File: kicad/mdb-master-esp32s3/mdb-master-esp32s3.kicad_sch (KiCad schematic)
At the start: 40 parts, among them J2 MDB_Connector, J3 Barrel_Jack, J5 Conn_02x10_Odd_Even, P1 USB_C_Plug_USB2.0, Q1 BC807, SW1 Reset, SW2 Boot, U1 ESP32-S3FH4R2, U2 TS1117B, Y1 40000hz

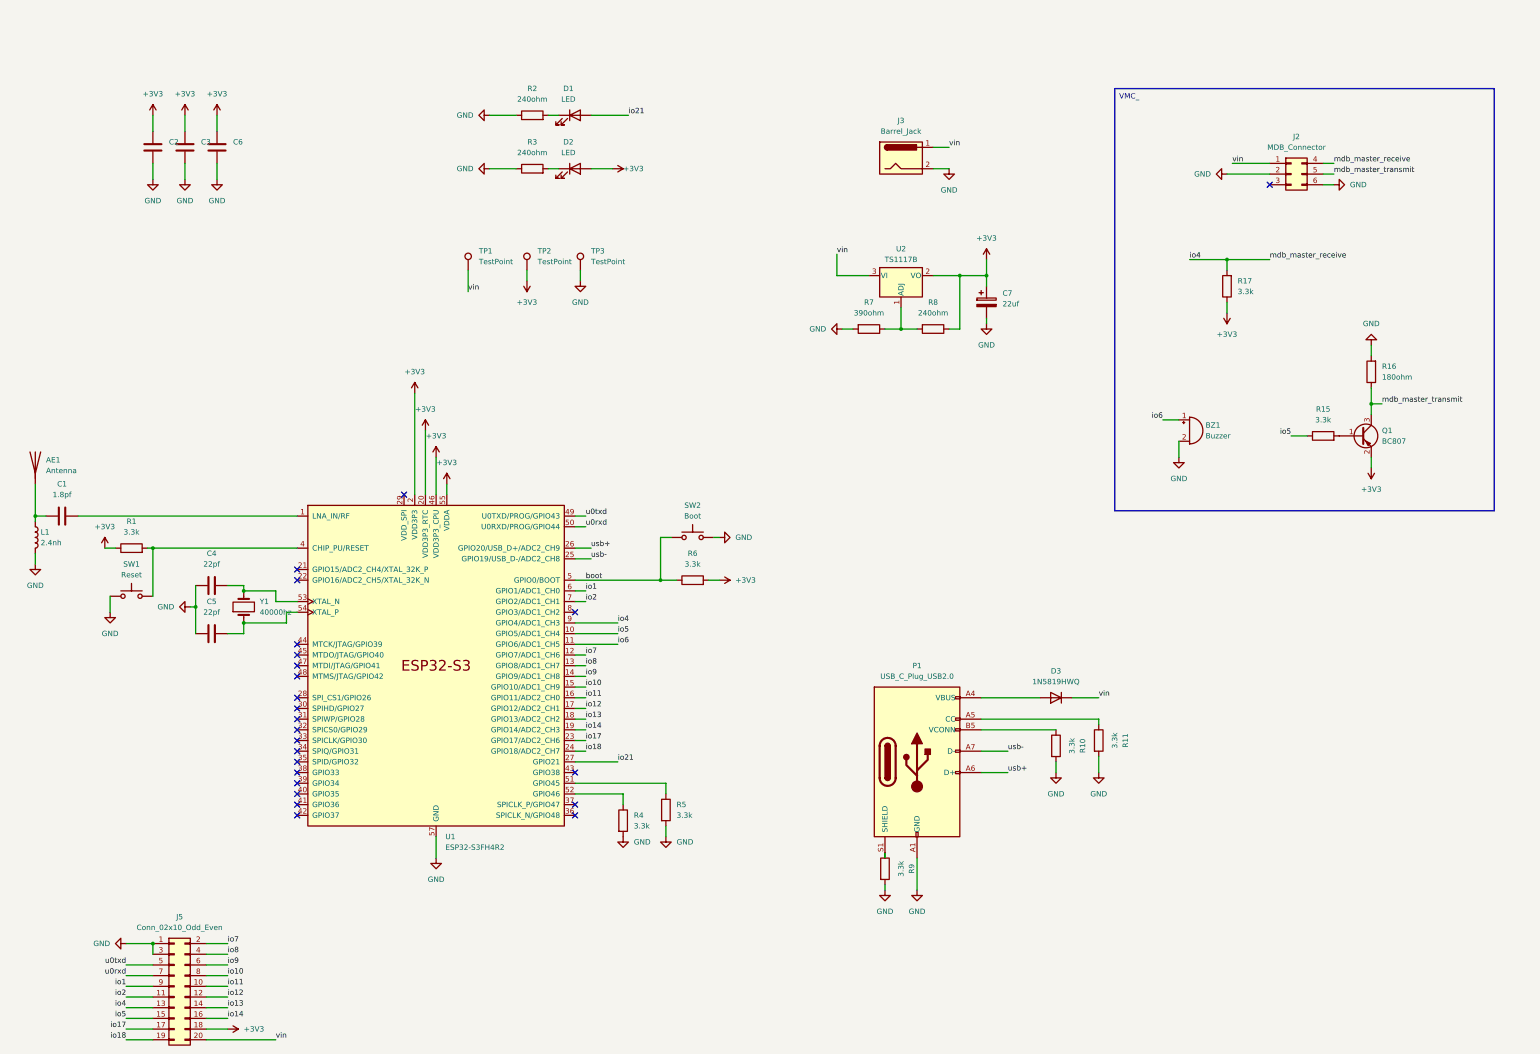
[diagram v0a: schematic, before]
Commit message: Refacting kicad pcb
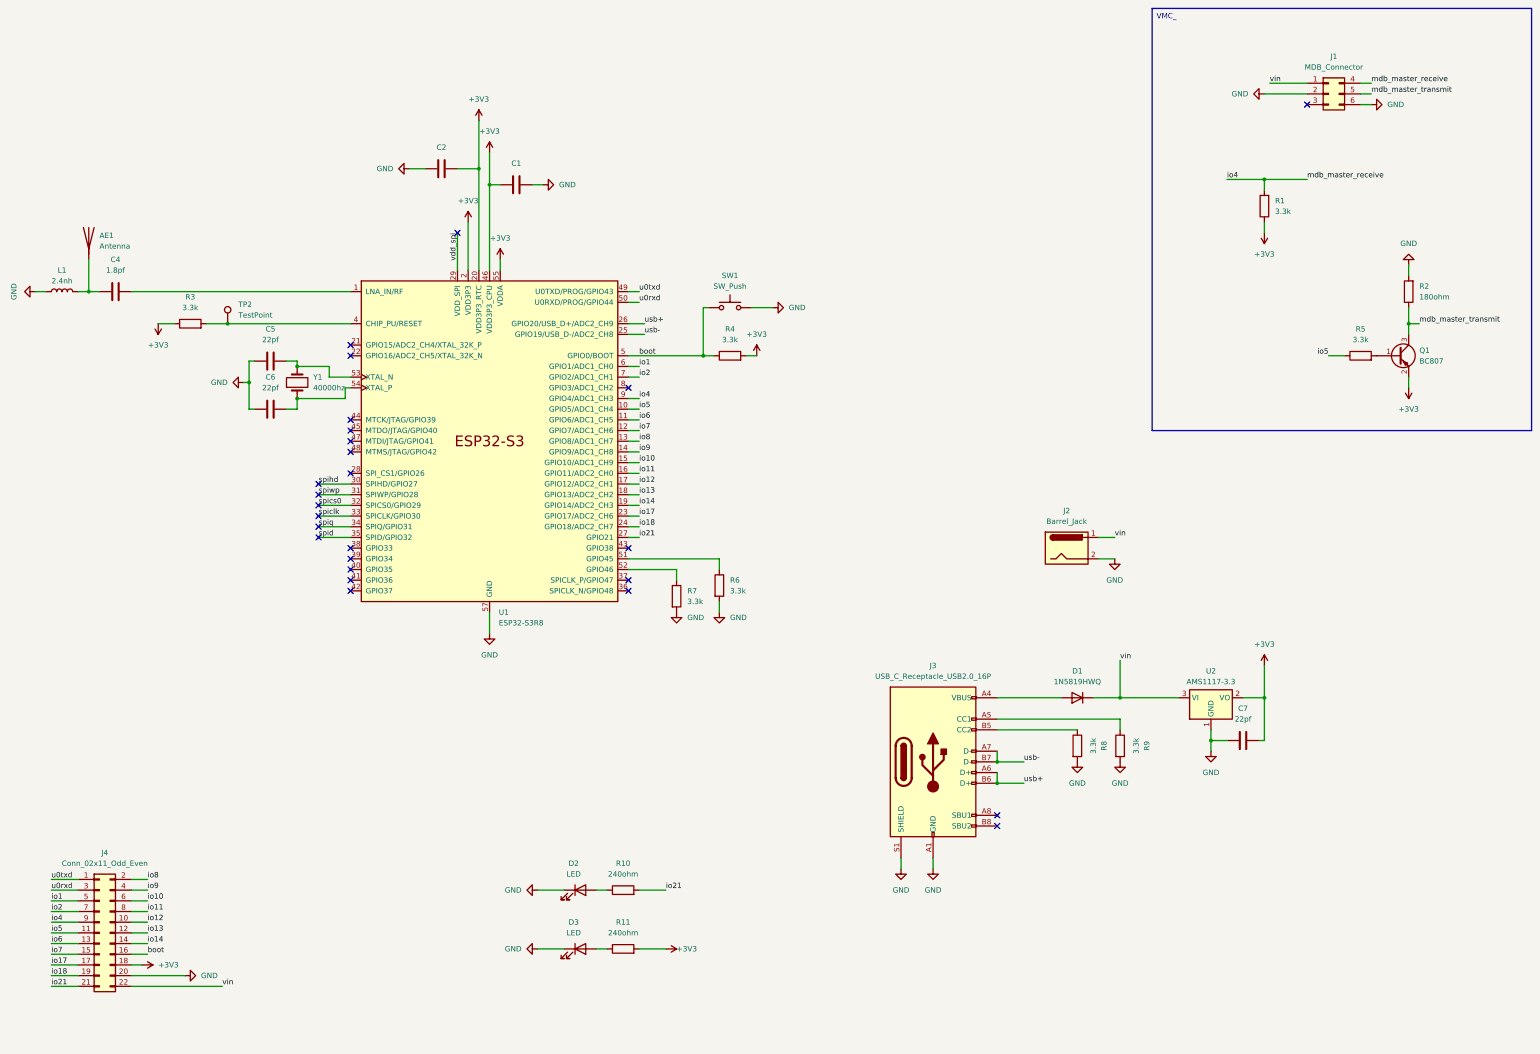
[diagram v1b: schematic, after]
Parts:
- removed BZ1: Buzzer, Buzzer_Beeper:Buzzer_12x9.5RM7.6, symbol Device:Buzzer
- removed C3: C, Capacitor_SMD:C_0603_1608Metric, symbol Device:C
- removed C7: 22uf, Capacitor_Tantalum_SMD:CP_EIA-3216-18_Kemet-A, symbol Device:C_Polarized
- removed D1: LED, LED_SMD:LED_0603_1608Metric, symbol Device:LED
- removed D3: 1N5819HWQ, Diode_SMD:D_SOD-123, symbol Device:D
- removed J2: MDB_Connector, Connector_Molex:Molex_Mini-Fit_Jr_5566-06A_2x03_P4.20mm_Vertical, symbol Connector_Generic:Conn_02x03_Top_Bottom
- removed J3: Barrel_Jack, Connector_BarrelJack:BarrelJack_Horizontal, symbol Connector:Barrel_Jack
- removed J5: Conn_02x10_Odd_Even, Connector_PinHeader_2.54mm:PinHeader_2x10_P2.54mm_Vertical, symbol Connector_Generic:Conn_02x10_Odd_Even
- removed P1: USB_C_Plug_USB2.0, Connector_USB:USB_C_Receptacle_G-Switch_GT-USB-7010ASV, symbol Connector:USB_C_Plug_USB2.0
- removed R15, R17: 3.3k, Resistor_SMD:R_0603_1608Metric, symbol Device:R
- removed R16: 180ohm, Resistor_SMD:R_0603_1608Metric, symbol Device:R
- removed SW2: Boot, Button_Switch_SMD:SW_Tactile_SPST_NO_Straight_CK_PTS636Sx25SMTRLFS, symbol Switch:SW_Push
- removed TP1, TP3: TestPoint, TestPoint:TestPoint_Pad_D1.0mm, symbol Connector:TestPoint
- removed U2: TS1117B, Package_TO_SOT_SMD:SOT-223-3_TabPin2, symbol Regulator_Linear:LM317_SOT-223
- added C7: 22pf, Capacitor_SMD:C_0603_1608Metric, symbol Device:C
- added D1: 1N5819HWQ, Diode_SMD:D_SOD-123, symbol Device:D
- added D3: LED, LED_SMD:LED_0603_1608Metric, symbol Device:LED
- added J1: MDB_Connector, Connector_Molex:Molex_Mini-Fit_Jr_5566-06A_2x03_P4.20mm_Vertical, symbol Connector_Generic:Conn_02x03_Top_Bottom
- added J2: Barrel_Jack, Connector_BarrelJack:BarrelJack_Horizontal, symbol Connector:Barrel_Jack
- added J3: USB_C_Receptacle_USB2.0_16P, Connector_USB:USB_C_Receptacle_G-Switch_GT-USB-7010ASV, symbol Connector:USB_C_Receptacle_USB2.0_16P
- added J4: Conn_02x11_Odd_Even, Connector_PinHeader_2.54mm:PinHeader_2x11_P2.54mm_Vertical, symbol Connector_Generic:Conn_02x11_Odd_Even
- added U2: AMS1117-3.3, Package_TO_SOT_SMD:SOT-223, symbol Regulator_Linear:AMS1117-3.3
- AE1: footprint RF_Antenna:Texas_SWRA117D_2.4GHz_Right -> RF_Antenna:Texas_SWRA117D_2.4GHz_Left
- C1: value 1.8pf -> C
- C4: value 22pf -> 1.8pf
- C6: value C -> 22pf
- R10, R11: value 3.3k -> 240ohm
- R2: value 240ohm -> 180ohm
- R3, R8: value 240ohm -> 3.3k
- R7: value 390ohm -> 3.3k
- SW1: value Reset -> SW_Push
- U1: value ESP32-S3FH4R2 -> ESP32-S3R8
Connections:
- net +3V3: now also C1.2, C2.1, R11.2, R3.1, R4.2, C7.2, J4.18 (Pin_18), U2.2 (VO); no longer C2.2, C6.2, D2.2 (A), R6.2, R8.1, TP2.1
- net GND: now also C1.1, C2.2, D2.1 (K), L1.1, R2.2, R6.2, R8.2, SW1.2, C7.1, D3.1 (K), J1.2 (Pin_2), J1.6 (Pin_6), J2.2, J3.A1 (GND), J3.A12 (GND), J3.B1 (GND), J3.B12 (GND), J3.S1 (SHIELD), J4.20 (Pin_20), U2.1 (GND); no longer C2.1, C4.1, L1.2, R10.2, R11.2, R2.1, R3.1, R4.2, R5.2, SW1.1
- net boot: now also R4.1, SW1.1, J4.16 (Pin_16); no longer R6.1
- net io1: now also J4.5 (Pin_5)
- net io10: now also J4.6 (Pin_6)
- net io11: now also J4.8 (Pin_8)
- net io12: now also J4.10 (Pin_10)
- net io13: now also J4.12 (Pin_12)
- net io14: now also J4.14 (Pin_14)
- net io17: now also J4.17 (Pin_17)
- net io18: now also J4.19 (Pin_19)
- net io2: now also J4.7 (Pin_7)
- net io21: now also R10.2, J4.21 (Pin_21)
- net io4: now also R1.2, J1.4 (Pin_4), J4.9 (Pin_9)
- net io5: now also R5.1, J4.11 (Pin_11)
- net io6: now also J4.13 (Pin_13)
- net io7: now also J4.15 (Pin_15)
- net io8: now also J4.2 (Pin_2)
- net io9: now also J4.4 (Pin_4)
- net mdb_master_transmit: now also R2.1, J1.5 (Pin_5)
- net u0rxd: now also J4.3 (Pin_3)
- net u0txd: now also J4.1 (Pin_1)
- net usb+: now also J3.A6 (D+), J3.B6 (D+)
- net usb-: now also J3.A7 (D-), J3.B7 (D-)
- net vin: now also D1.1 (K), J1.1 (Pin_1), J2.1, J4.22 (Pin_22), U2.3 (VI)
- net at Q1.1 (B): now also R5.2
- net at R3.2: now also TP2.1, U1.4 (CHIP_PU/RESET); no longer D2.1 (K)
- net at U1.51 (GPIO45): now also R6.1; no longer R5.1
- net at U1.1 (LNA_IN/RF): now also C4.2; no longer C1.2
- net vdd_spi: now reaches U1.29 (VDD_SPI)
- net spihd: now reaches U1.30 (SPIHD/GPIO27)
- net spiwp: now reaches U1.31 (SPIWP/GPIO28)
- net spics0: now reaches U1.32 (SPICS0/GPIO29)
- net spiclk: now reaches U1.33 (SPICLK/GPIO30)
- net spiq: now reaches U1.34 (SPIQ/GPIO31)
- net spid: now reaches U1.35 (SPID/GPIO32)
- net at U1.52 (GPIO46): now also R7.1; no longer R4.1
- net at U1.53 (XTAL_N), Y1.2: now also C5.2; no longer C4.2
- net at U1.54 (XTAL_P), Y1.1: now also C6.2; no longer C5.2
- net at R9.1: now also J3.A5 (CC1)
- net at R10.1: now also D2.2 (A)
- net at R11.1: now also D3.2 (A)
- new net: AE1.1 (A), C4.1, L1.2
- new net: D1.2 (A), J3.A4 (VBUS), J3.A9 (VBUS), J3.B4 (VBUS), J3.B9 (VBUS)
- new net: J3.B5 (CC2), R8.1
- no-connect marks 24 -> 26
